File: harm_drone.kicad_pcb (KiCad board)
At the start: 4 copper layers, 100 x 40 mm, 62 parts, among them IC1 Microcontroller, IC2 USB Hub, IC3 SRAM, IC4 LDO, J1 SYS_DEBUG, J2 2-Port USB, J3 2-Port USB, J4 SD_Card, J5 SPI2, J6 SPI1, J7 XT60-M, U1 LMR51430, U2 EEPROM

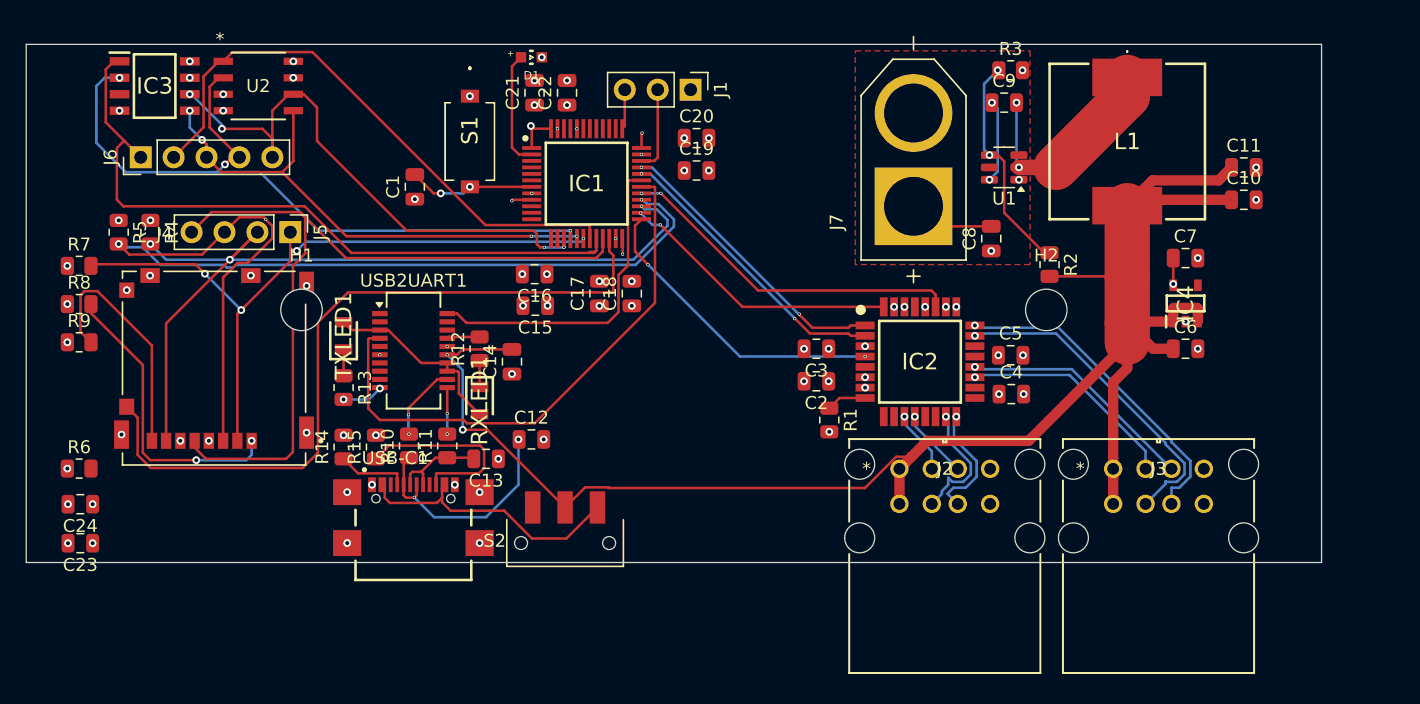
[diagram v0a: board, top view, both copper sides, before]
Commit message: final changes
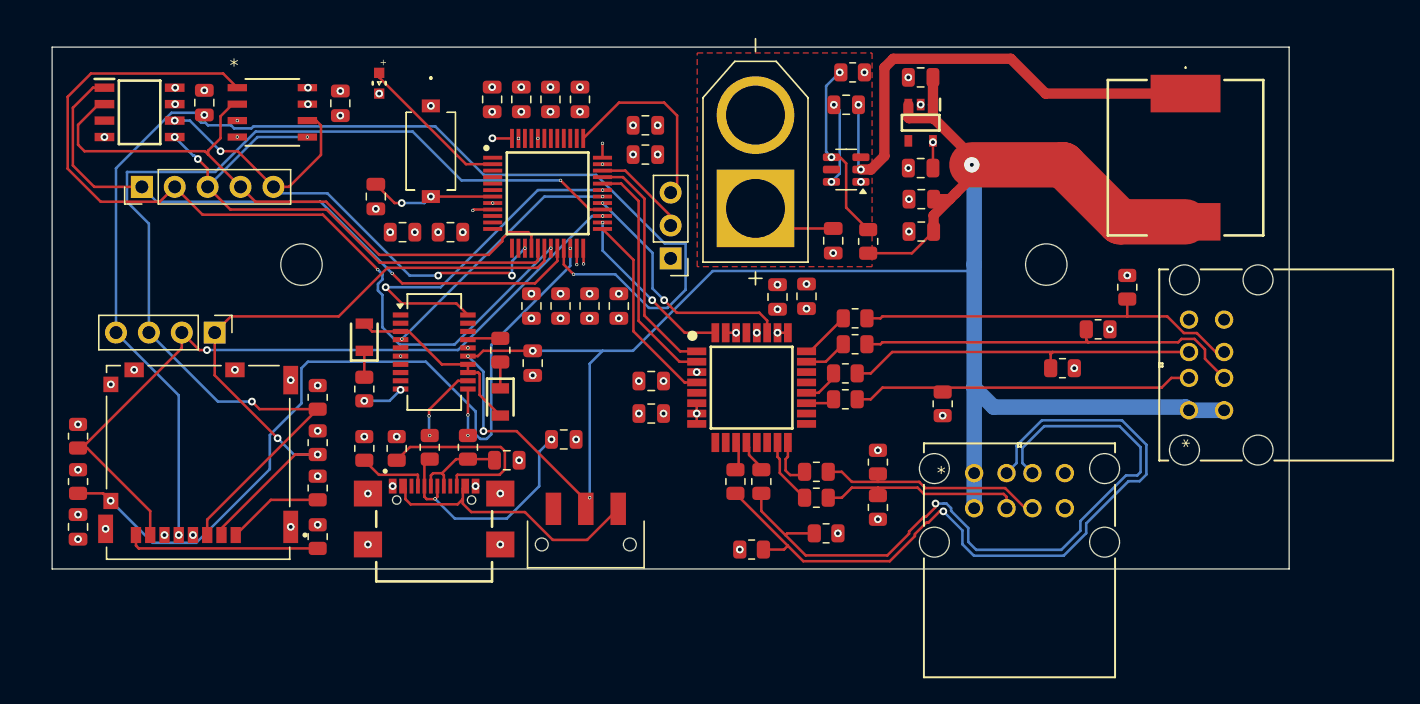
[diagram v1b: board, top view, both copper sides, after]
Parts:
- removed the C15 at (132.8, 98.2)
- removed the C16 at (132.8, 95.7)
- removed the C17 at (137.8, 97.2)
- removed the C18 at (140.2, 97.2)
- removed the C19 at (145.2, 87.7)
- removed the C20 at (145.2, 85.2)
- removed the C21 at (132.7, 81.7)
- removed the C22 at (135.2, 81.7)
- removed the C23 at (97.7, 116.5)
- added C10: 0.1uF, Capacitor_SMD:C_0805_2012Metric, F.Cu at (132.5, 98.2)
- added C11: 4.7uF, Capacitor_SMD:C_0805_2012Metric, F.Cu at (134.8, 98.2)
- added C12: 0.1uF, Capacitor_SMD:C_0805_2012Metric, F.Cu at (141.3, 86.5)
- added C13: 4.7uF, Capacitor_SMD:C_0805_2012Metric, F.Cu at (141.3, 84.2)
- added C2: 0.1uF, Capacitor_SMD:C_0805_2012Metric, F.Cu at (136.2, 82.2)
- added C25: 2.2uF, Capacitor_SMD:C_0805_2012Metric, F.Cu at (117.8, 82.5)
- added C26: 2.2uF, Capacitor_SMD:C_0805_2012Metric, F.Cu at (107.2, 82.5)
- added C3: 0.1uF, Capacitor_SMD:C_0805_2012Metric, F.Cu at (134.0, 82.2)
- added C4: 10nF, Capacitor_SMD:C_0805_2012Metric, F.Cu at (126.2, 92.5)
- added C5: 0.1uF, Capacitor_SMD:C_0805_2012Metric, F.Cu at (129.5, 82.2)
- added C6: 0.1uF, Capacitor_SMD:C_0805_2012Metric, F.Cu at (122.5, 92.5)
- added C7: 4.7uF, Capacitor_SMD:C_0805_2012Metric, F.Cu at (131.7, 82.2)
- added C8: 0.1uF, Capacitor_SMD:C_0805_2012Metric, F.Cu at (137.0, 98.2)
- added C9: 0.1uF, Capacitor_SMD:C_0805_2012Metric, F.Cu at (139.2, 98.2)
- added R10: 15kOhm, Resistor_SMD:R_0805_2012Metric, F.Cu at (164.2, 105.8)
- added R11: 15kOhm, Resistor_SMD:R_0805_2012Metric, F.Cu at (155.2, 115.8)
- added R12: 15kOhm, Resistor_SMD:R_0805_2012Metric, F.Cu at (173.5, 103.0)
- added R13: 15kOhm, Resistor_SMD:R_0805_2012Metric, F.Cu at (159.2, 113.8)
- added R14: 15kOhm, Resistor_SMD:R_0805_2012Metric, F.Cu at (176.2, 100.0)
- added R15: 15kOhm, Resistor_SMD:R_0805_2012Metric, F.Cu at (159.2, 110.2)
- added R16: 15kOhm, Resistor_SMD:R_0805_2012Metric, F.Cu at (178.5, 96.8)
- added R2: 27ohm, Resistor_SMD:R_0805_2012Metric, F.Cu at (150.2, 111.8)
- added R3: 27ohm, Resistor_SMD:R_0805_2012Metric, F.Cu at (154.5, 113.0)
- added R4: 27ohm, Resistor_SMD:R_0805_2012Metric, F.Cu at (154.5, 111.0)
- added R5: 27ohm, Resistor_SMD:R_0805_2012Metric, F.Cu at (156.7, 105.4)
- added R6: 27ohm, Resistor_SMD:R_0805_2012Metric, F.Cu at (156.7, 103.4)
- added R7: 27ohm, Resistor_SMD:R_0805_2012Metric, F.Cu at (157.5, 101.2)
- added R8: 27ohm, Resistor_SMD:R_0805_2012Metric, F.Cu at (157.5, 99.2)
- added R9: 15kOhm, Resistor_SMD:R_0805_2012Metric, F.Cu at (149.5, 117.0)
- C24: value 0.1uF -> 2.2uF
- R1: value 2kOhm -> 27ohm
- R21: renamed from R6; value 27 -> 27ohm
- moved C18 29.3 mm to (162.6, 80.5), turned to 180 degrees
- moved C23 25.4 mm to (162.6, 92.5), turned to 180 degrees
- moved C22 24.9 mm to (162.6, 90.0), turned to 180 degrees
- moved IC3 24.8 mm to (162.6, 84.0), turned to -90 degrees
- moved R24 23.7 mm to (116.0, 116.0), turned to -90 degrees
- moved R23 23.3 mm to (116.0, 112.2), turned to -90 degrees
- moved R22 22.9 mm to (116.0, 108.8), turned to -90 degrees
- moved C19 21.6 mm to (162.6, 87.5), turned to 180 degrees
- moved R20 20.0 mm to (116.0, 105.2)
- moved C17 18.6 mm to (151.5, 97.5), turned to 90 degrees
- moved C16 17.5 mm to (153.7, 97.5), turned to 90 degrees
- moved R19 16.7 mm to (97.5, 108.2)
- moved R17 14.1 mm to (158.5, 93.2)
- moved IC2 13.2 mm to (149.5, 104.5)
- moved J1 13.1 mm to (143.2, 94.5), turned to 180 degrees
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- renumbered C2 to C14, C3 to C15, C4 to C16, C5 to C17, C6 to C18, C7 to C19, C8 to C20, C9 to C21, C10 to C22, C11 to C23, C12 to C27, C13 to C28, C14 to C29, IC4 to IC3, IC3 to IC4, J7 to J4, J4 to J5, J5 to J6, J6 to J7, R2 to R17, R3 to R18, R4 to R19, R5 to R20, R7 to R22, R8 to R23, R9 to R24, R10 to R25, R11 to R26, R12 to R27, R13 to R28, R14 to R29, R15 to R30
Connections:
- C24 pad 1: GND -> 3V3
- C24 pad 2: 3V3 -> GND
- IC1 pad 1: 3V3 -> unconnected-(IC1-VBAT-Pad1)
- IC2 pad 8: Net-(IC2-BUSPWR) -> GND
- J2 pad 2: /USB/D1- -> /USB/J2_D1-
- J2 pad 3: /USB/D1+ -> /USB/J2_D1+
- J2 pad 6: /USB/D2- -> /USB/J2_D2-
- J2 pad 7: /USB/D2+ -> /USB/J2_D2+
- J3 pad 2: /USB/D3- -> /USB/J3_D1-
- J3 pad 3: /USB/D3+ -> /USB/J3_D1+
- J3 pad 6: /USB/D4- -> /USB/J3_D2-
- J3 pad 7: /USB/D4+ -> /USB/J3_D2+
- R1 pad 1: Net-(IC2-BUSPWR) -> /USB/D1-
- R1 pad 2: GND -> /USB/J2_D1-
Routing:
- net /USB/J2_D1-: track 0.00 -> 59.0 mm, vias 0 -> 1
- net /USB/J2_D1+: track 0.00 -> 56.1 mm, vias 0 -> 1
- net SPI CLOCK 2: track 62.8 -> 96.8 mm, vias 0 -> 2
- net /USB/J3_D2-: track 0.00 -> 30.5 mm
- net /USB/J3_D2+: track 0.00 -> 30.1 mm
- net 5V: track 133.5 -> 161.3 mm, vias 2 -> 5
- net /USB/J3_D1+: track 0.00 -> 27.6 mm
- net /USB/J3_D1-: track 0.00 -> 26.3 mm
- net CS EEPROM: track 44.3 -> 69.5 mm, vias 0 -> 2
- net RXD_USB2SERIAL: track 42.7 -> 20.1 mm, vias 0 -> 2
- net /USB/D4-: track 25.4 -> 3.40 mm, vias 1 -> 0
- net Net-(U1-SW): track 17.2 -> 38.8 mm
- net /USB/D4+: track 25.3 -> 3.89 mm, vias 1 -> 0
- net /USB/J2_D2+: track 0.00 -> 17.5 mm
- net /USB/J2_D2-: track 0.00 -> 15.9 mm
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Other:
- board size 100 x 40 mm -> 95.5 x 40.3 mm
